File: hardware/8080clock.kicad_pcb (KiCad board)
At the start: 2 copper layers, 199.7 x 119.9 mm, 105 parts, among them J1 4840-2201, J10 POWER OUTPUT, J2 2032 battery, J6 POWER INPUT, J7 1WIRE, J8 SPEAKER, J9 BME280, M1 MountingHole_3.2mm_M3.0, M2 MountingHole_3.2mm_M3.0, M3 MountingHole_3.2mm_M3.0, M4 MountingHole_3.2mm_M3.0, M5 MountingHole_3.2mm_M3.0, M6 MountingHole_3.2mm_M3.0, M7 MountingHole_3.2mm_M3.0, M8 MountingHole_3.2mm_M3.0, Q1 IRF4905, Q2 IRF4905, Q3 BC547, SW1 Button 1, SW2 Button 2, SW3 Button 3, SW4 RESET, U1 NE555N, U10 Intel 8255A / КР580ВВ55А, U11 PCF8563P, U12 Intel 8080 / КР580ВМ80, U2 L7905ACV, U3 TPS54260, U5 Intel 8224 / КР580ГФ24, U6 Intel 8238 / КР580ВК38, U7 CY62256L-70PC, U8 27C256 / КР573РФ8, U9 74LS04 / К555ЛН1, Y1 32MHZ, Y2 32.768

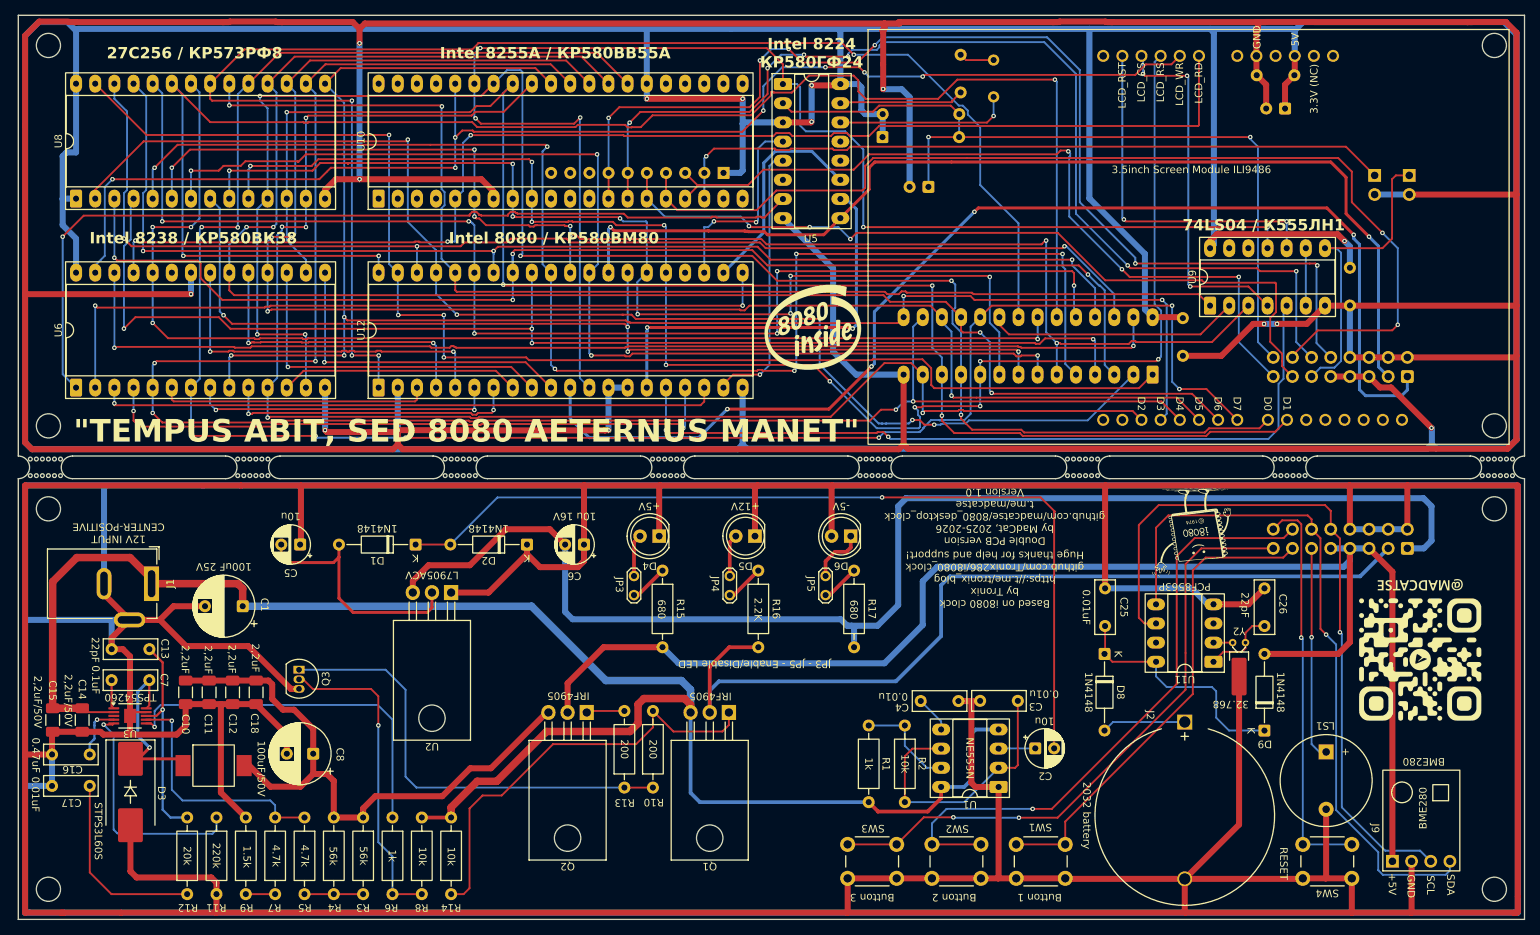
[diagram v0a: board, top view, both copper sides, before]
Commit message: Clock Update
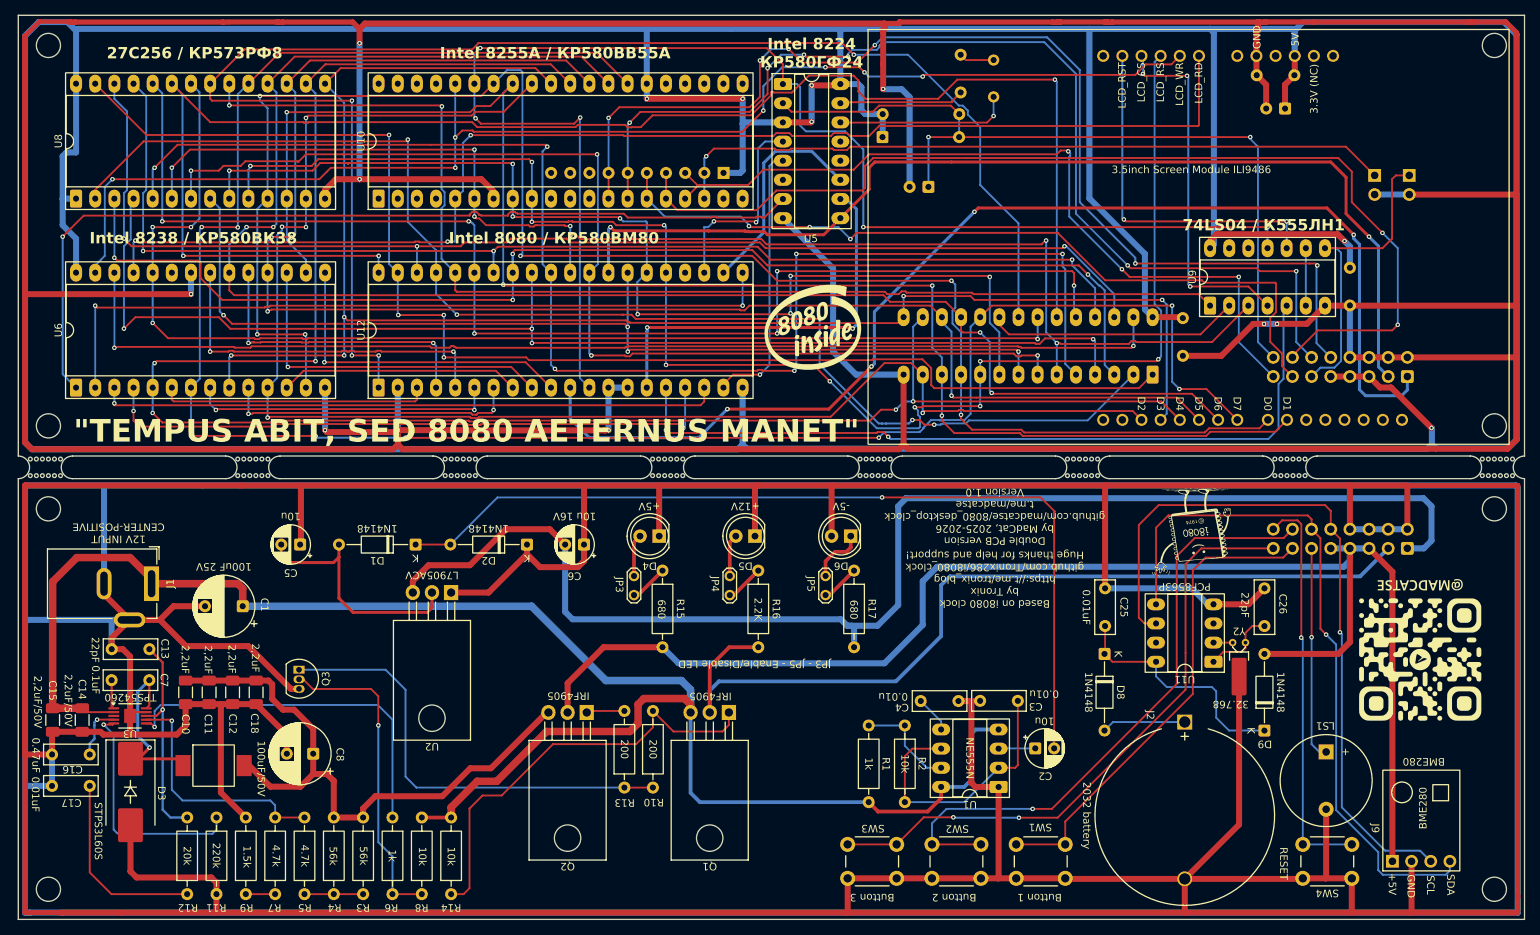
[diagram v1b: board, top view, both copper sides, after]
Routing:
- net GND: track 2282.6 -> 2281.9 mm
